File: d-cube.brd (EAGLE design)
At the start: 75.9 x 53.3 mm, 63 parts, among them IC1 74AC86D, IC2 SFH6156, IC3 SFH6156, IC4 ISO7220M, IC5 ISO7221M, IC7 NXE2, IC8 ADUM3160, U3 COMPLEMENTARY

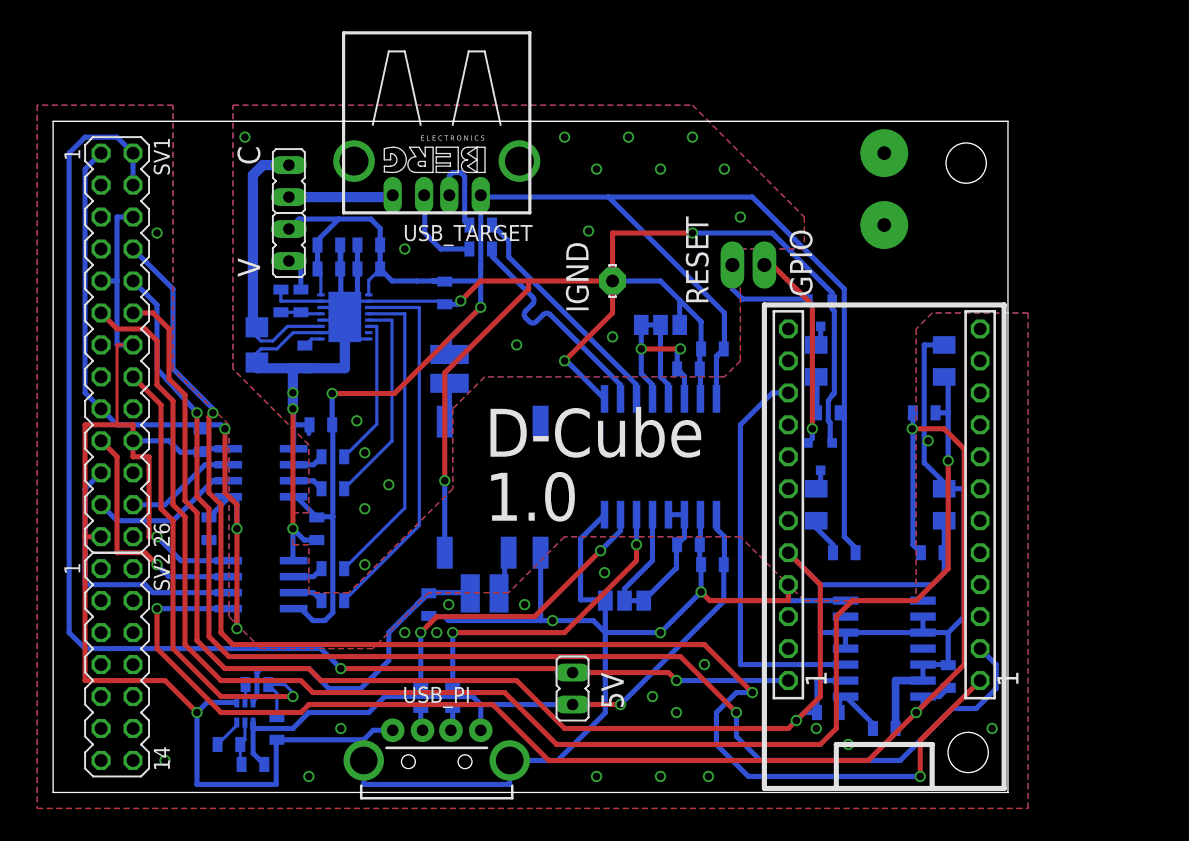
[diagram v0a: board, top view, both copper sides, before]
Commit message: Update to 2.1
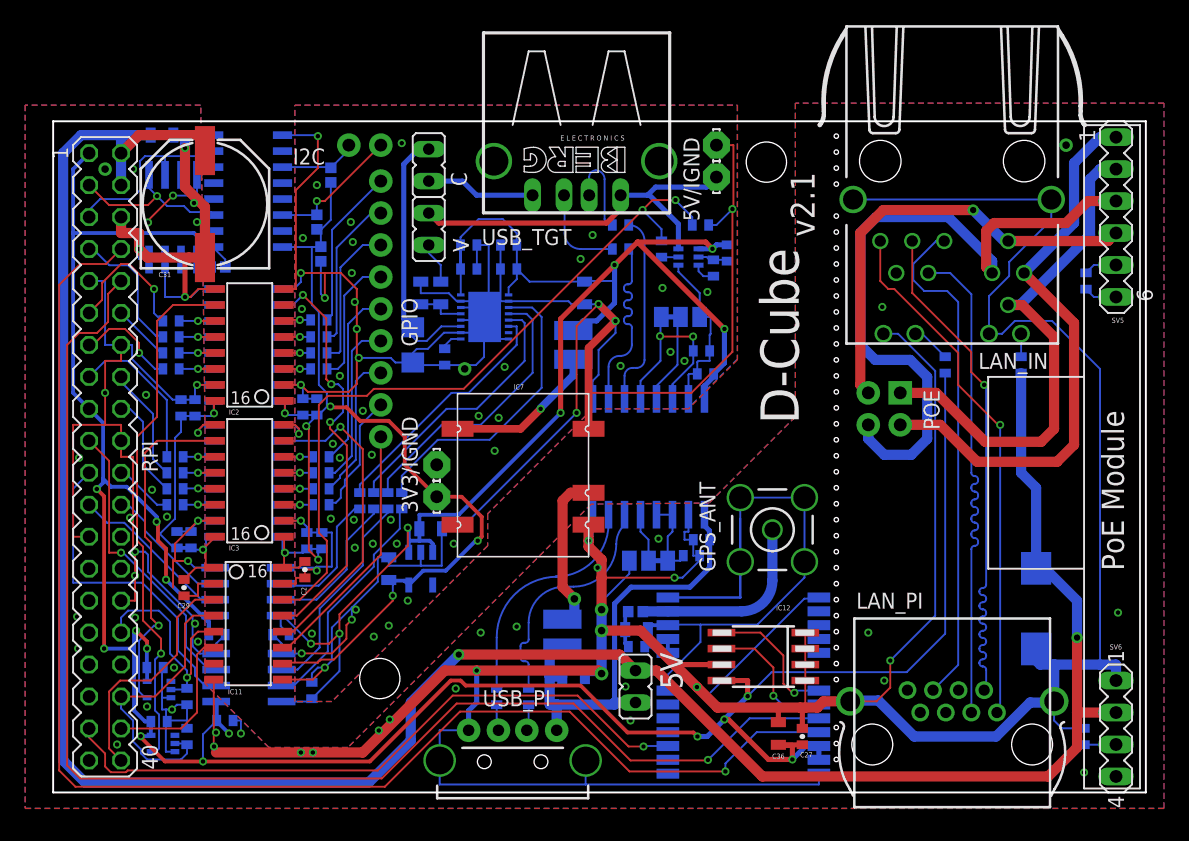
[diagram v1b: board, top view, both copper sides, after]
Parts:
- removed IGND: LSP10, solpad:LSP10
- removed J1: (no value), SparkFun-Connectors:1X02_LONGPADS
- removed NS1, NS2: (no value), con-samtec:SSW-112-02-S-S
- removed Q1, Q2: (no value), transistors:SOT-23
- removed SV1: (no value), con-lstb:MA13-2
- removed SV2: (no value), con-lstb:MA07-2
- removed U3: COMPLEMENTARY, mos:SOT-363
- removed USB_TARGET: PN87520-S, con-berg:PN87520-S
- added C20, C21, C22, C23, C24, C25, C26, C27, C29, C3, C5: 0.1u, SparkFun-Passives:0402-CAP
- added C30: 470u, rcl:CT7343
- added C31: 1000uF, SparkFun-Capacitors:PANASONIC_G
- added C32: 0.1u, SparkFun-Passives:0805
- added C33, C34: 0.1uF, SparkFun-Capacitors:0402
- added C35: 10n, SparkFun-Passives:0805
- added C36: 10uF, SparkFun-Capacitors:0805
- added C37, C38: 1.0uF, SparkFun-Capacitors:0805
- added GPIO: (no value), SparkFun-Connectors:1X09_NO_SILK
- added GPS_ANT: BU-SMA-V, con-coax:BU-SMA-V
- added I2C: (no value), SparkFun-Connectors:1X02_NO_SILK
- added IC10, IC11, IC9: SI8640AB-B-IS1, silabslbr:SO-16
- added IC12: 24AA32ASM, microchip:SO-08M
- added IC13: I2C EEPROM, SparkFun-IC-Memory:SO08-EIAJ
- added IC14: NEO-M8, ubloxLib:NEO-M8
- added IC15: MIC550X-YM5, borkedlabs-powerics:SOT23-5-DBV
- added IC16: COMPLEMENTARY, mos:SOT-363
- added IC17, IC18: 74LVC1G04, SparkFun-DigitalIC:SOT353
- added L3: 27nH, SparkFun-Coils:0402
- added LAN_IN: SI-52008-F, con-pulse:POE
- added LAN_PI: 0446200002, con-molex:0446200002
- added POE: (no value), my-con:2X02_NO_SILK
- added R21, R22, R23, R24, R29, R30, R31, R32: 100, SparkFun-Passives:0402-RES
- added R25, R26, R27, R28, R35: 100k, SparkFun-Passives:0402-RES
- added R33, R34: 10k, SparkFun-Passives:0402-RES
- added R36: 220, SparkFun-Passives:0402-RES
- added R37: 470, SparkFun-Passives:0402-RES
- added R38: 10, SparkFun-Passives:0402-RES
- added R40, R41: 100k, SparkFun-Resistors:0402
- added RPI: (no value), con-lstb:MA20-2
- added SV5: (no value), con-lstb:MA06-1
- added SV6: (no value), con-lstb:MA04-1
- added TP_3V3, TP_IGND, TP_IGND1, TP_VCC: LSP10, solpad:LSP10
- added U$1, U$2: (no value), tugraz:TU-LOGO-SMALL
- added USB_TGT: PN87520-S, con-berg:PN87520-S
- C1, C2: value 100n -> 0.1u; device SparkFun-Passives:0805 -> SparkFun-Passives:0402-CAP
- C10, C11, C12, C13, C14, C15, C16, C17, C18, C19, C7, C8, C9: device SparkFun-Passives:0805 -> SparkFun-Passives:0402-CAP
- IC1: value 74AC86D -> SI8605; device 74xx-eu:SO14 -> silabslbr:SO-16
- IC2, IC3: value SFH6156 -> SI8640AB-B-IS1; device optocoupler:SFH -> silabslbr:SO-16
- R1: value 3k3 -> 10k; device SparkFun-Passives:0805 -> SparkFun-Passives:0402-RES
- R10, R11, R12, R13, R15, R17, R18, R19, R20, R6, R7, R9: device SparkFun-Passives:0805 -> SparkFun-Passives:0402-RES
- R2, R3: value 470 -> 100k; device SparkFun-Passives:0805 -> SparkFun-Passives:0402-RES
- R4, R5: value 10k -> 100k; device SparkFun-Passives:0805 -> SparkFun-Passives:0402-RES
- moved IC1 62.2 mm to (15.6, 47.8)
- moved C1 58.1 mm to (8.10, 9.92)
- moved R9 55.4 mm to (53.6, 42.9), turned to 90 degrees
- moved R7 54.0 mm to (52.5, 41.7), turned to 90 degrees
- moved R6 52.3 mm to (51.4, 45.1), turned to 0 degrees
- moved R5 52.1 mm to (21.1, 37.5), turned to 180 degrees
- moved C2 51.8 mm to (20.0, 17.7), flipped to the top, turned to 270 degrees
- moved IC2 51.7 mm to (15.6, 35.6), flipped to the top, turned to 90 degrees
- moved IC3 51.1 mm to (15.6, 24.8), flipped to the top, turned to 90 degrees
- moved R4 48.5 mm to (21.1, 36.2), turned to 180 degrees
- moved R20 47.2 mm to (48.3, 43.2), turned to 270 degrees
- moved R2 44.2 mm to (21.1, 33.7), turned to 180 degrees
- moved R3 40.8 mm to (21.1, 34.9), turned to 180 degrees
- moved R1 39.9 mm to (82.1, 40.6), turned to 90 degrees
- moved C13 17.0 mm to (18.1, 12.5)
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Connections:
- removed net 5V_SW: C4.1, L1.P$1, U3.3
- removed net GPIO1: IC1.2, IC2.4, NS2.5, R1.1, R5.1, SV1.12
- removed net GPIO2: IC3.4, R4.1, SV1.11
- removed net GPIO3: R20.1, R6.2, SV1.16
- removed net GPIO_EDGE: IC1.3, NS2.10
- removed net GPIO_LP: C1.1, IC1.1, R1.2
- removed net GPIO_TARGET: J1.1, Q1.1
- removed net RESET_TARGET: J1.2, Q2.1
- removed net VCCIO: NS2.3
- new net !EN_BLOCK1: IC17.4, IC2.10
- new net !EN_BLOCK2: IC18.4, IC3.10
- new net AIN: IC1.4
- new net AOUT: IC1.5
- new net B1C1: R21.2, RPI.11
- new net B1C2: R22.2, RPI.7
- new net B1C3: R23.2, RPI.12
- new net B1C4: R24.2, RPI.13
- new net B2C1: R29.2, RPI.15
- new net B2C2: R30.2, RPI.16
- new net B2C3: R31.2, RPI.18
- new net B2C4: R32.2, RPI.22
- new net BIN: IC1.12
- new net BOUT: IC1.13
- new net BSCL: I2C.1, IC1.11, R41.1
- new net BSDA: I2C.2, IC1.14, R40.1
- new net CP1: R1.2, SV5.5
- new net CP2: R1.1, SV5.6
- new net CT: LAN_IN.2
- new net EN_BLOCK1: IC11.4, IC17.2, R34.2, RPI.36
- new net EN_BLOCK2: IC11.5, IC18.2, R33.2, RPI.32
- new net GPS_SIG: GPS_ANT.1, IC14.11, L3.1
- new net GSCL: IC12.6, IC14.19
- new net GSDA: IC12.5, IC14.18
- new net I_B1C1: GPIO.4, R2.2
- new net I_B1C2: GPIO.3, R3.2
- new net I_B1C3: GPIO.2, R4.2
- new net I_B1C4: GPIO.1, R5.2
- new net I_B2C1: GPIO.8, R25.2
- new net I_B2C2: GPIO.7, R26.2
- new net I_B2C3: GPIO.6, R27.2
- new net I_B2C4: GPIO.5, R28.2
- new net I_EN_BLOCK1: IC10.10, IC11.13
- new net I_EN_BLOCK2: IC11.12, IC9.10
- new net I_PWR_SW: IC11.14, R20.1, R6.2
- new net I_RST_SW: GPIO.9, IC11.11
- new net N$10: LAN_IN.G+, R37.2
- new net N$13: IC10.11, IC2.6, R5.1
- new net N$15: IC10.13, IC2.4, R3.1
- new net N$21: IC10.6, IC2.11, R21.1
- new net N$23: IC3.6, IC9.11, R28.1
- new net N$24: IC3.5, IC9.12, R27.1
- new net N$25: IC3.4, IC9.13, R26.1
- new net N$26: IC3.14, IC9.3, R32.1
- new net N$27: IC3.13, IC9.4, R31.1
- new net N$28: IC3.12, IC9.5, R30.1
- new net N$29: IC3.11, IC9.6, R29.1
- new net N$30: IC14.8, IC14.9, R38.2
- new net N$32: C35.1, L3.2, R38.1
- new net N$6: IC10.3, IC2.14, R24.1
- new net N$7: IC10.4, IC2.13, R23.1
- new net N$9: LAN_IN.Y+, R36.2
- new net OADJ: R35.1, SV6.3
- new net PPS: IC14.3, RPI.37
- new net PWR_SW: IC11.3, RPI.40
- new net RST_SW: IC11.6, RPI.38
- new net RX+: LAN_IN.4, LAN_PI.3
- new net RX-: LAN_IN.5, LAN_PI.6
- new net SCL: IC1.6, IC13.6, RPI.5
- new net SDA: IC1.3, IC13.5, RPI.3
- new net TX+: LAN_IN.1, LAN_PI.1
- new net TX-: LAN_IN.3, LAN_PI.2
- new net VCC/2: C2.1, C21.1, C24.1, C3.1, C34.1, C38.1, C5.1, IC1.16, IC10.16, IC11.10, IC11.16, IC15.5, IC2.1, IC3.1, IC9.16, R40.2, R41.2, TP_3V3.MP
- new net VCC_SW: IC16.3, TP_VCC.MP, USB_TGT.1, V.1
- new net VINA+: LAN_IN.10, POE.2, SV5.1
- new net VINA-: LAN_IN.11, POE.1, SV5.2
- new net VINB+: LAN_IN.8, POE.4, SV5.3
- new net VINB-: LAN_IN.9, POE.3, SV5.4
- net +3V3: now also C1.1, C20.1, C22.1, C23.1, C25.1, C26.1, C27.1, C29.1, C33.1, C36.1, IC1.1, IC10.1, IC11.1, IC12.8, IC13.8, IC14.22, IC14.23, IC17.5, IC18.5, IC2.16, IC3.16, IC9.1, R36.1, RPI.1, RPI.17; no longer C2.1, IC1.14, R4.2, R5.2, SV1.1, SV1.17
- net +5V: now also C30.+, C31.+, C32.1, R37.1, RPI.2, RPI.4, SV6.2; no longer NS2.1, SV1.2, SV1.4
- net CSB: now also RPI.24; no longer SV1.24
- net D+_OUT_TERM: now also USB_TGT.3; no longer USB_TARGET.3
- net D-_OUT_TERM: now also USB_TGT.2; no longer USB_TARGET.2
- net GND: now also C20.2, C22.2, C23.2, C25.2, C26.2, C27.2, C29.2, C30.-, C31.-, C32.2, C33.2, C35.2, C36.2, GPS_ANT.2, GPS_ANT.3, GPS_ANT.4, GPS_ANT.5, IC1.8, IC10.2, IC10.8, IC11.2, IC11.8, IC12.1, IC12.2, IC12.3, IC12.4, IC12.7, IC13.1, IC13.2, IC13.3, IC13.4, IC14.10, IC14.12, IC14.13, IC14.24, IC14.7, IC17.3, IC18.3, IC2.15, IC2.9, IC3.15, IC3.9, IC9.2, IC9.8, LAN_IN.G-, LAN_IN.M1, LAN_IN.M2, LAN_IN.Y-, LAN_PI.S@1, LAN_PI.S@2, R33.1, R34.1, R35.2, RPI.14, RPI.20, RPI.25, RPI.30, RPI.34, RPI.39, RPI.6, RPI.9, SV6.1; no longer C2.2, IC1.10, IC1.12, IC1.13, IC1.4, IC1.5, IC1.7, IC1.9, IC2.3, IC3.3, NS2.4, R6.1, SV1.14, SV1.20, SV1.25, SV1.6, SV1.9, U3.1
- net GNDA: now also C2.2, C21.2, C24.2, C3.2, C34.2, C37.2, C38.2, C5.2, IC1.9, IC10.15, IC10.9, IC11.15, IC11.9, IC15.2, IC16.1, IC2.2, IC2.8, IC3.2, IC3.8, IC9.15, IC9.9, R6.1, TP_IGND.MP, TP_IGND1.MP; no longer IGND.MP, Q1.2, Q2.2
- net MISO: now also RPI.21; no longer SV1.21
- net MOSI: now also RPI.19; no longer SV1.19
- net N$11: now also IC10.5, IC2.12, R22.1; no longer IC2.1, R2.2
- net N$12: now also IC3.3, IC9.14, R25.1; no longer IC3.1, R3.2
- net N$14: now also IC10.12, IC2.5, R4.1; no longer IC3.2, Q2.3
- net N$2: now also IC10.14, IC2.3, R2.1; no longer IC2.2, Q1.3
- net N$3: now also IC16.2; no longer U3.2
- net N$4: now also IC16.5; no longer U3.5
- net N$8: now also IC16.6; no longer U3.6
- net RXD: now also IC14.20, RPI.10; no longer NS1.2, SV1.10
- net SCLK: now also RPI.23; no longer SV1.23
- net TXD: now also IC14.21, RPI.8; no longer NS1.1, SV1.8
- net V-: now also USB_TGT.4; no longer USB_TARGET.4
- net VBUS: now also C4.1, L1.P$1; no longer R9.2, U3.4
- net VCC: now also C37.1, IC15.1, IC15.3, IC16.4, R9.2; no longer R2.1, R3.1, USB_TARGET.1, V.1
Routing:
- net GND: track 261.8 -> 504.2 mm, vias 24 -> 56
- net GPIO2: track 121.7 -> 0.00 mm, vias 1 -> 0
- net GPIO1: track 120.0 -> 0.00 mm, vias 1 -> 0
- net VCC/2: track 0.00 -> 90.9 mm, vias 0 -> 7
- net +5V: track 105.5 -> 195.5 mm
- net GNDA: track 182.2 -> 254.9 mm, vias 24 -> 53
- net +3V3: track 175.1 -> 243.8 mm, vias 6 -> 17
- net I_PWR_SW: track 0.00 -> 58.7 mm, vias 0 -> 2
- net VINB+: track 0.00 -> 55.3 mm
- net PPS: track 0.00 -> 52.7 mm, vias 0 -> 1
- net VINA+: track 0.00 -> 45.4 mm
- net VINA-: track 0.00 -> 41.9 mm
- net TX+: track 0.00 -> 41.9 mm, vias 0 -> 1
- net !EN_BLOCK1: track 0.00 -> 41.7 mm, vias 0 -> 1
- net TX-: track 0.00 -> 40.9 mm, vias 0 -> 1
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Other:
- board size 75.9 x 53.3 mm -> 86.8 x 53.3 mm
- board text added: "3V3/IGND"
- board text added: "5V/IGND"
- board text added: "IC14"
- board text added: "L1"
- board text added: "L2"
- board text added: "PoE Module"
- board text added: "v2.1"
- board text removed: "1.0"
- board text removed: "GPIO"
- board text removed: "RESET"
